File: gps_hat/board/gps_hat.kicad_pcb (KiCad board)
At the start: 2 copper layers, 36.5 x 63.5 mm, 14 parts, among them IC1 MTK3339, J1 Conn_02x10_Odd_Even, J2 U.FL-R-SMT(10)

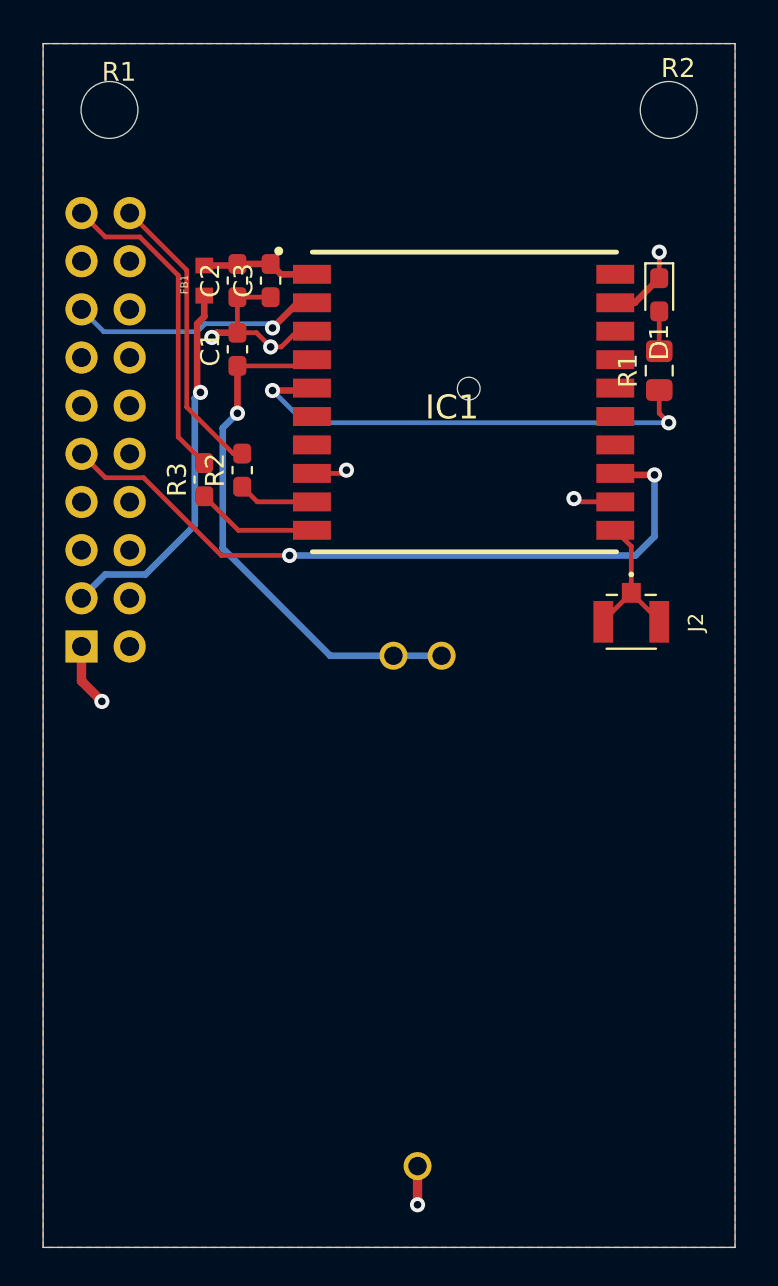
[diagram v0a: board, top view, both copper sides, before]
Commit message: Fixed PCB Layout
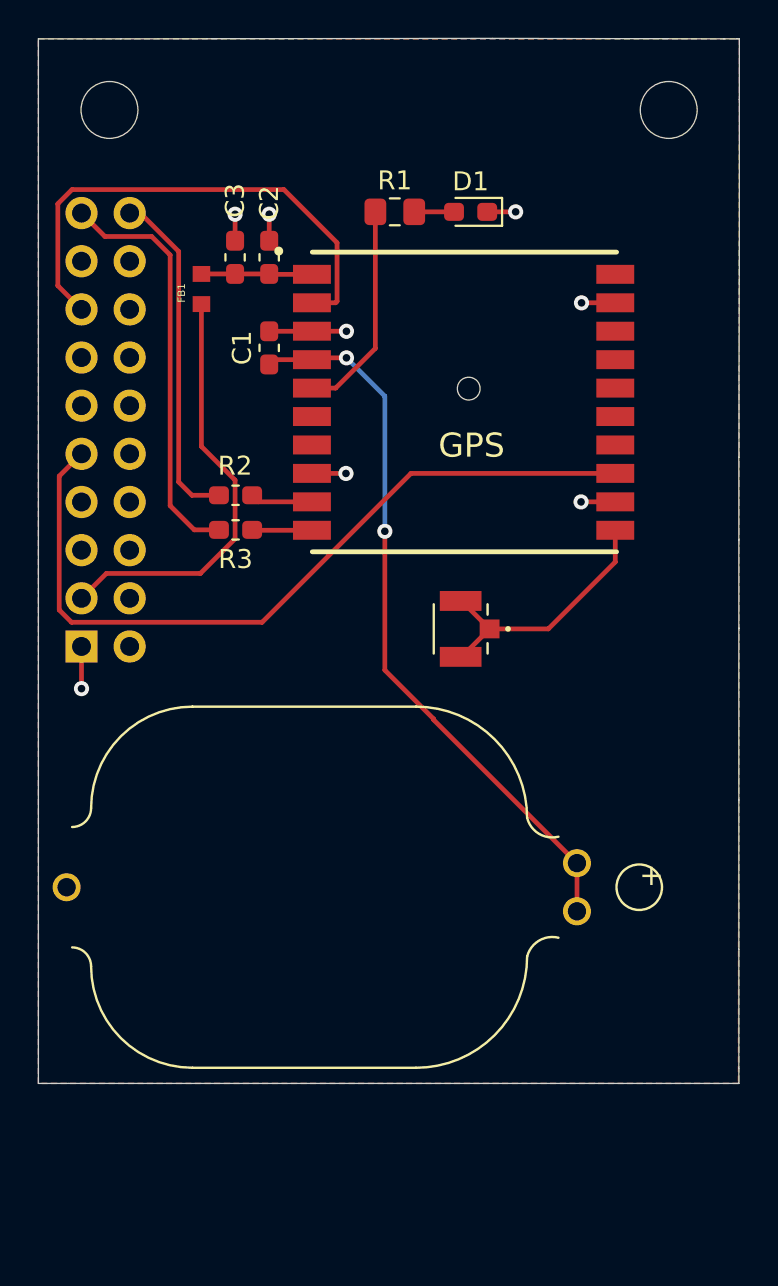
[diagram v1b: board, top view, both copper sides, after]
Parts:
-  : renamed from R2
-  : renamed from R1
-  : renamed from BT1; moved to F.Cu
-  : renamed from J2
- moved R1 16.3 mm to (148.1, 65.4), turned to 0 degrees
- moved D1 10.9 mm to (152.1, 65.4), turned to 180 degrees
- moved   9.01 mm to (151.5, 87.4), turned to 180 degrees
- moved   5.20 mm to (144.2, 101.0), turned to 180 degrees
- moved R3 3.12 mm to (139.7, 82.2), turned to 180 degrees
- moved C3 2.24 mm to (139.6, 67.8), turned to 270 degrees
- moved C2 2.08 mm to (141.4, 67.8), turned to 270 degrees
- moved C1 1.68 mm to (141.4, 72.5)
- moved R2 1.37 mm to (139.7, 80.3), turned to 180 degrees
- moved FB1 0.47 mm to (137.8, 69.4)
- renumbered IC1 to GPS
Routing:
- net Net-(IC1-Pad5): track 25.8 -> 11.6 mm, vias 2 -> 0
- net /NRESET: track 13.5 -> 27.5 mm, vias 1 -> 0
- net Net-(BT1-Pad+1): track 27.9 -> 38.9 mm, vias 1 -> 2
- net GND: track 23.4 -> 16.8 mm, vias 7 -> 8
- net Net-(IC1-Pad11): track 7.92 -> 14.0 mm
- net /TX: track 16.9 -> 21.9 mm
- net Net-(IC1-Pad10): track 6.89 -> 3.16 mm
- net /1PPS: track 38.4 -> 41.7 mm, vias 2 -> 0
- net /RX: track 15.4 -> 18.0 mm
- net +3V3: track 20.0 -> 22.5 mm, vias 1 -> 0
- net Net-(IC1-Pad9): track 4.01 -> 3.30 mm
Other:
- board size 36.5 x 63.5 mm -> 37 x 55.1 mm
